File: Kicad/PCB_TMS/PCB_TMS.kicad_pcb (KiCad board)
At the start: 2 copper layers, 30 parts, among them J1 Conn_ARM_JTAG_SWD_10, SW1 SW_DPDT_x2, U1 STM32F030F4Px, U2 MCP9700T-ETT, U3 M24C01-FDW, Y1 20MHz

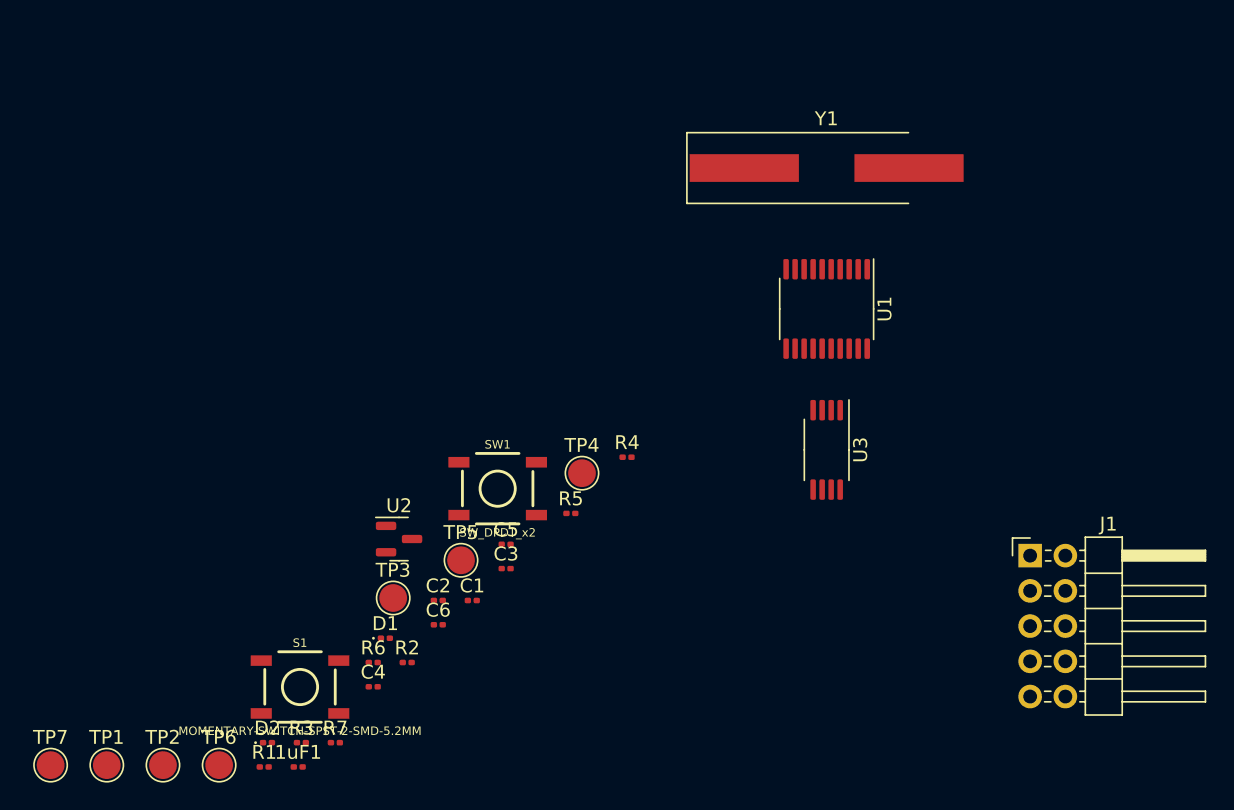
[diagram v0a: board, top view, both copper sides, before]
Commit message: Routage v1
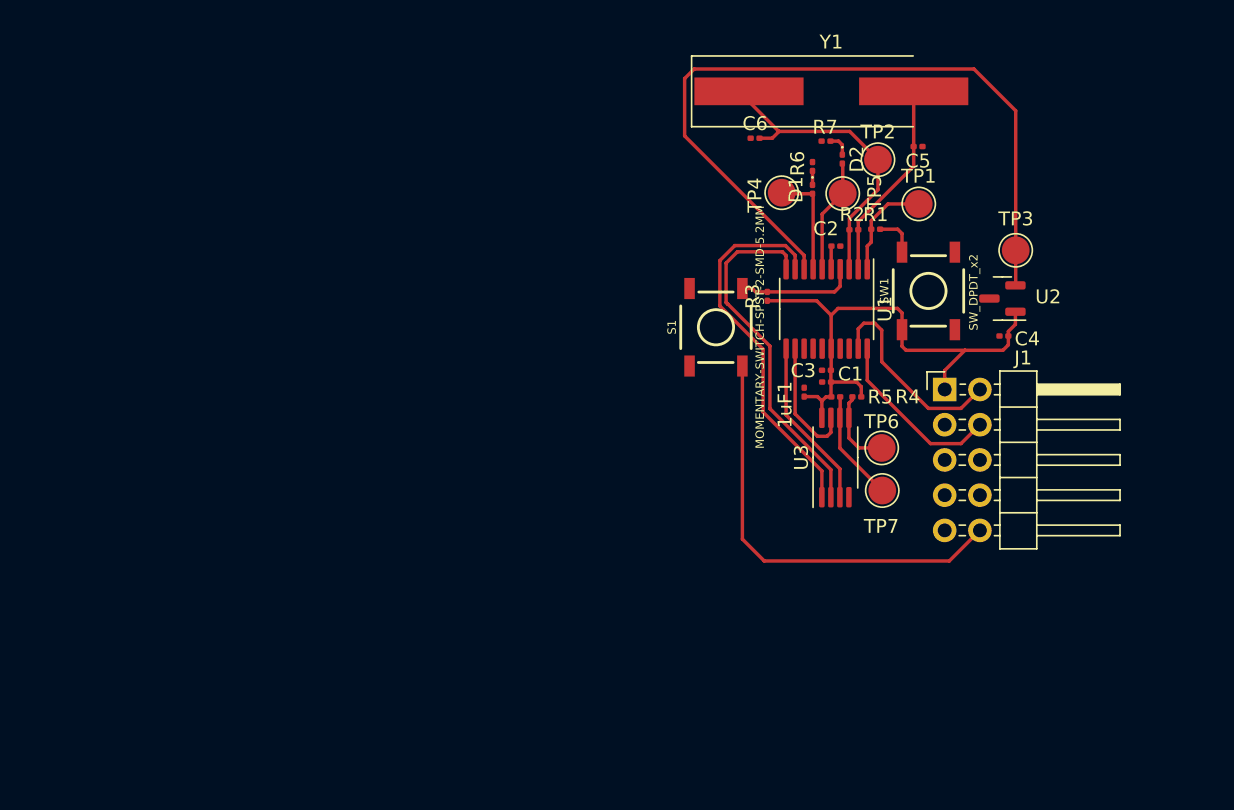
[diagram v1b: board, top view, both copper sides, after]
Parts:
- moved TP1 71.2 mm to (169.2, 76.2)
- moved TP2 67.5 mm to (166.3, 73.1)
- moved TP7 63.1 mm to (166.6, 96.9)
- moved D2 59.1 mm to (163.7, 73.0), turned to -90 degrees
- moved R1 58.7 mm to (166.1, 78.1)
- moved R7 56.0 mm to (162.5, 71.7), turned to 180 degrees
- moved TP6 53.0 mm to (166.5, 93.8)
- moved C4 52.0 mm to (175.3, 85.8)
- moved TP3 51.4 mm to (176.2, 79.6), turned to 180 degrees
- moved R6 47.8 mm to (161.5, 73.5), turned to 90 degrees
- moved U2 46.8 mm to (175.2, 83.1), turned to 180 degrees
- moved R3 46.5 mm to (158.3, 82.9), turned to 90 degrees
- moved 1uF1 45.4 mm to (160.9, 89.8), turned to 90 degrees
- moved R2 44.8 mm to (164.5, 78.1), turned to 180 degrees
- moved D1 44.7 mm to (161.5, 75.2), turned to -90 degrees
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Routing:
- net TEMP: track 0.00 -> 55.3 mm
- net +3.3V: track 0.00 -> 40.9 mm
- net RST: track 0.00 -> 39.7 mm
- net E0: track 0.00 -> 27.3 mm
- net E1: track 0.00 -> 25.8 mm
- net Net-(C6-Pad2): track 0.00 -> 22.1 mm
- net SWDIO/TMS: track 0.00 -> 14.8 mm
- net Net-(C5-Pad2): track 0.00 -> 14.5 mm
- net SWCLM/TCK: track 0.00 -> 12.9 mm
- net E2: track 0.00 -> 12.3 mm
- net WC: track 0.00 -> 9.12 mm
- net LED0: track 0.00 -> 8.25 mm
- net SCL: track 0.00 -> 8.02 mm
- net LED1: track 0.00 -> 7.71 mm
- net BOOT: track 0.00 -> 7.55 mm
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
